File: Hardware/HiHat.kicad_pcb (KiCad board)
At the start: 2 copper layers, 63.5 x 105.4 mm, 45 parts, among them J1 Inputs, J2 Output, J3 IDC power connector, Q1 BC549, Q2 BC549, Q3 BC549, Q4 BC549, U1 TL074

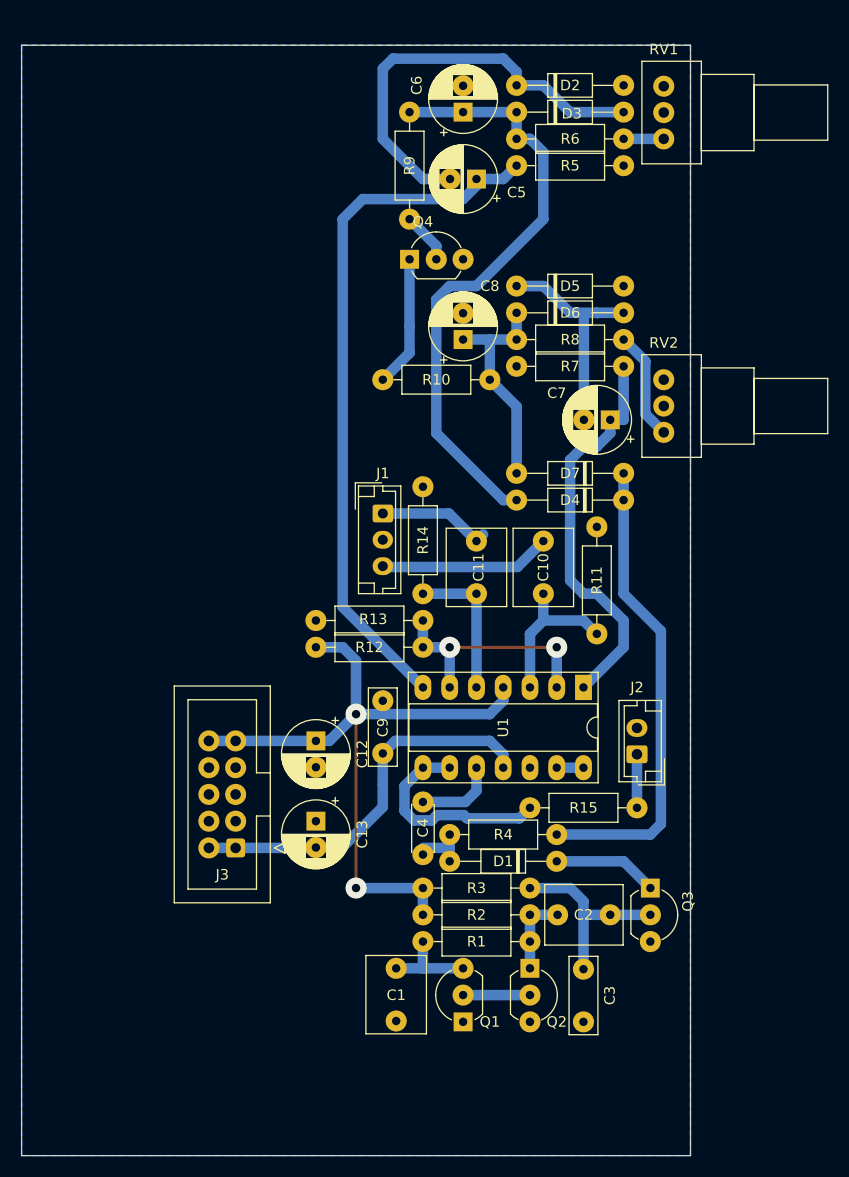
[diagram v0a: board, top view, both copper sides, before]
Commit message: PCB routing
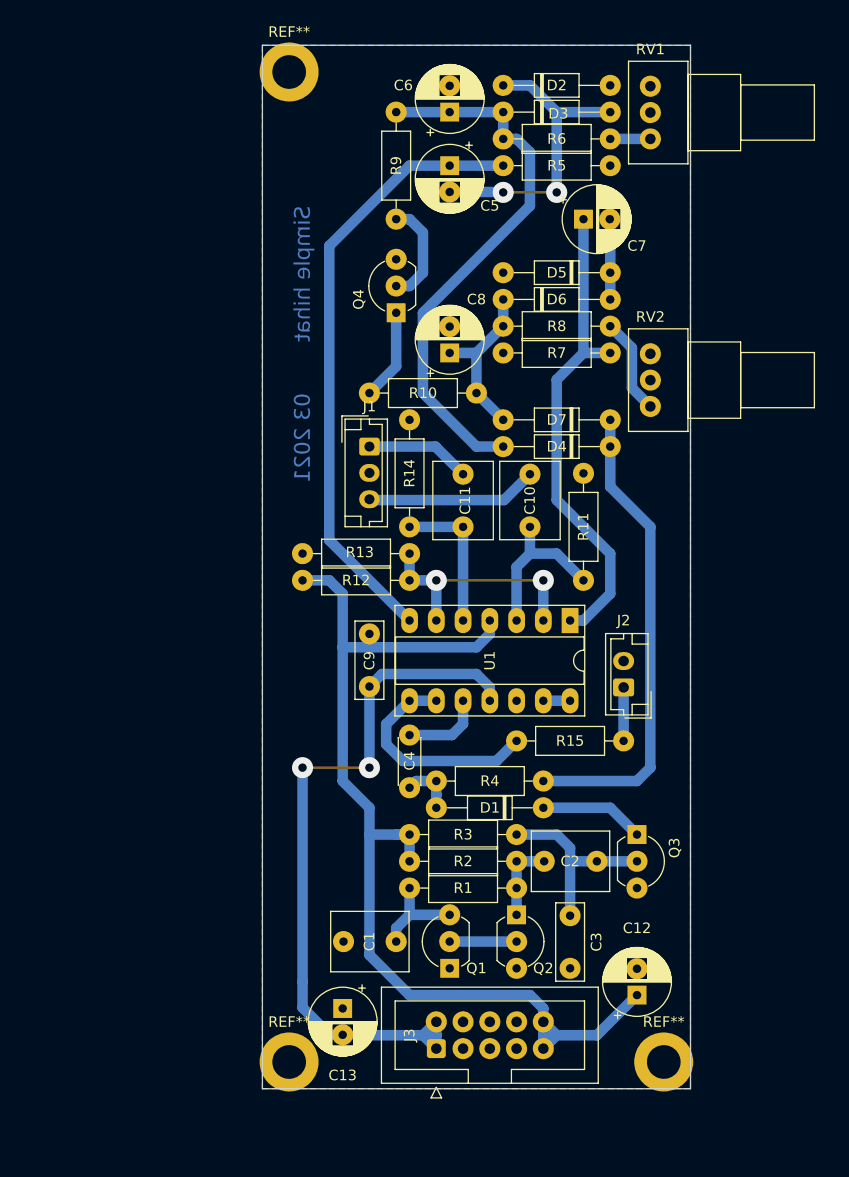
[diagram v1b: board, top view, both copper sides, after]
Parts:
- added REF**: MountingHole_3.2mm_M3_DIN965_Pad, MountingHole:MountingHole_3.2mm_M3_DIN965_Pad, F.Cu at (111.8, 166.4)
- added REF**: MountingHole_3.2mm_M3_DIN965_Pad, MountingHole:MountingHole_3.2mm_M3_DIN965_Pad, F.Cu at (76.2, 72.4)
- added REF**: MountingHole_3.2mm_M3_DIN965_Pad, MountingHole:MountingHole_3.2mm_M3_DIN965_Pad, F.Cu at (76.2, 166.4)
- moved C12 38.9 mm to (109.2, 160.0), turned to 90 degrees
- moved J3 26.9 mm to (90.2, 165.1), turned to 90 degrees
- moved C7 19.2 mm to (104.1, 86.4), turned to 0 degrees
- moved C13 18.0 mm to (81.3, 161.3)
- moved D5 8.98 mm to (106.7, 91.4), turned to 180 degrees
- moved R15 6.48 mm to (108.0, 135.9)
- moved C11 6.48 mm to (92.7, 115.6)
- moved C9 6.48 mm to (83.8, 125.7)
- moved R14 6.48 mm to (87.6, 115.6)
- moved C10 6.48 mm to (99.1, 115.6)
- moved U1 6.48 mm to (102.9, 124.5)
- moved C4 6.48 mm to (87.6, 140.3)
- moved J1 6.48 mm to (83.8, 108.0)
- moved R13 6.48 mm to (87.6, 118.1)
- moved J2 6.48 mm to (108.0, 130.8)
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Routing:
- net +12V: track 66.9 -> 100.8 mm, vias 2 -> 0
- net -12V: track 36.9 -> 69.2 mm, vias 0 -> 2
- net Net-(C7-Pad2): track 21.4 -> 7.64 mm
- net Net-(C5-Pad2): track 40.7 -> 29.0 mm, vias 0 -> 2
- net Net-(C5-Pad1): track 66.6 -> 58.4 mm
- net Net-(C7-Pad1): track 38.5 -> 46.1 mm
- net Net-(C6-Pad1): track 58.4 -> 52.6 mm
- net Net-(C8-Pad1): track 21.4 -> 16.1 mm
- net Net-(Q4-Pad2): track 4.86 -> 9.94 mm
- net Net-(Q4-Pad1): track 12.5 -> 8.67 mm
- net Net-(R8-Pad2): track 10.5 -> 9.20 mm
- net Net-(R15-Pad2): track 20.4 -> 21.4 mm
- net CHtrig: track 10.9 -> 9.98 mm
- net Net-(C1-Pad1): track 8.89 -> 9.42 mm
- net Net-(C10-Pad1): track 15.0 -> 15.5 mm
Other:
- board size 63.5 x 105.4 mm -> 40.6 x 99.1 mm
- board text added: "03 2021"
- board text added: "Simple hihat"
